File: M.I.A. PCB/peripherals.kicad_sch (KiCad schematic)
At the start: 69 parts, among them J10 Conn_01x03, J11 Conn_01x03, J12 MSD-4-A, J13 Conn_01x04_Socket, J14 Conn_01x03, J15 Conn_01x03, J16 Conn_01x03, J17 Conn_01x03, J18 Conn_01x04_Socket, J19 Conn_01x04_Socket, J20 Screw_Terminal_01x02, J21 Screw_Terminal_01x02, J22 Screw_Terminal_01x02, J23 Screw_Terminal_01x02, J24 Conn_01x04_Socket, J25 Conn_01x08_Socket, J26 Conn_01x04_Socket, J27 Conn_01x02_Socket, J28 Conn_01x04_Socket, J29 Conn_01x02_Socket, J30 Conn_01x02_Socket, J31 Conn_01x02_Socket, J32 Screw_Terminal_01x02, J33 Screw_Terminal_01x02, J6 Conn_01x04_Socket, J7 Conn_01x03, J8 Conn_01x03, J9 Conn_01x04_Socket, Q1 AO3400A, Q2 AO3400A, Q3 AO3400A, Q4 AO3400A, U15 74AHC541

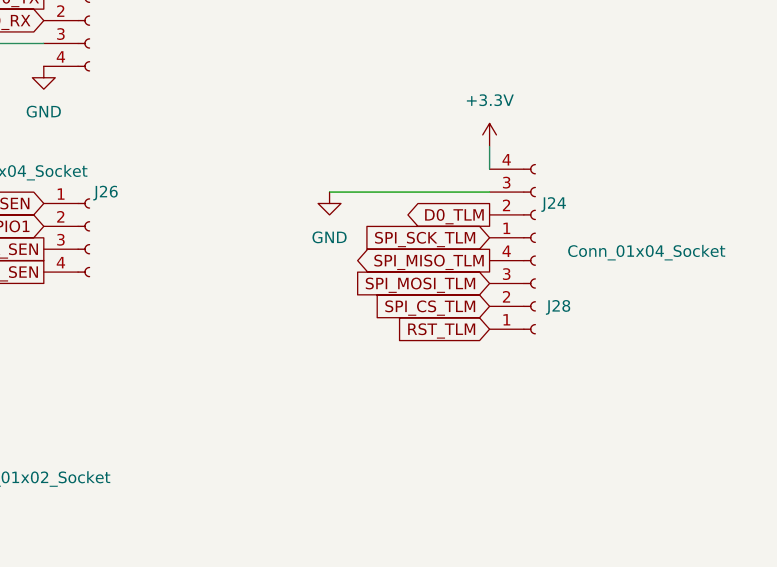
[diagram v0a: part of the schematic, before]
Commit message: Final Fixes, impedances, silkscreen etc
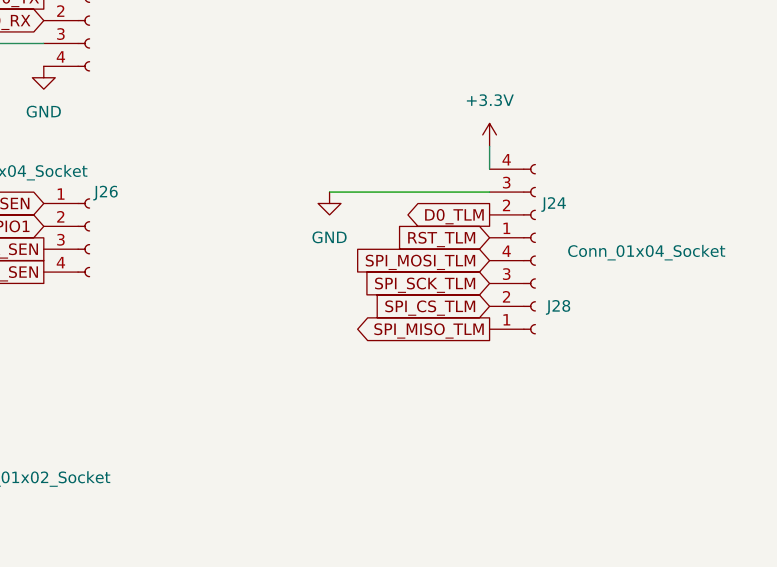
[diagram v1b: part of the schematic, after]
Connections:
- net RST_TLM: now also J24.1 (Pin_1); no longer J28.1 (Pin_1)
- net SPI_MISO_TLM: now also J28.1 (Pin_1); no longer J28.4 (Pin_4)
- net SPI_MOSI_TLM: now also J28.4 (Pin_4); no longer J28.3 (Pin_3)
- net SPI_SCK_TLM: now also J28.3 (Pin_3); no longer J24.1 (Pin_1)
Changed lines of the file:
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@@
 	(global_label "SPI_SCK_TLM"
 		(shape input)
-		(at 313.69 130.81 180)
-		(fields_autoplaced yes)
-		(effects
-			(font
-				(size 1.27 1.27)
-			)
-			(justify right)
-		)
-		(property "Intersheetrefs" "${INTERSHEET_REFS}"
-			(at 298.4887 130.81 0)
+		(at 313.69 135.89 180)
+		(fields_autoplaced yes)
+		(effects
+			(font
+				(size 1.27 1.27)
+			)
+			(justify right)
+		)
+		(property "Intersheetrefs" "${INTERSHEET_REFS}"
+			(at 299.7587 135.89 0)
 			(effects
 				(font
@@
 	(global_label "SPI_MISO_TLM"
 		(shape output)
-		(at 313.69 133.35 180)
-		(fields_autoplaced yes)
-		(effects
-			(font
-				(size 1.27 1.27)
-			)
-			(justify right)
-		)
-		(property "Intersheetrefs" "${INTERSHEET_REFS}"
-			(at 297.642 133.35 0)
+		(at 313.69 140.97 180)
+		(fields_autoplaced yes)
+		(effects
+			(font
+				(size 1.27 1.27)
+			)
+			(justify right)
+		)
+		(property "Intersheetrefs" "${INTERSHEET_REFS}"
+			(at 297.642 140.97 0)
 			(effects
 				(font
@@
 	(global_label "SPI_MOSI_TLM"
 		(shape input)
-		(at 313.69 135.89 180)
-		(fields_autoplaced yes)
-		(effects
-			(font
-				(size 1.27 1.27)
-			)
-			(justify right)
-		)
-		(property "Intersheetrefs" "${INTERSHEET_REFS}"
-			(at 297.642 135.89 0)
+		(at 313.69 133.35 180)
+		(fields_autoplaced yes)
+		(effects
+			(font
+				(size 1.27 1.27)
+			)
+			(justify right)
+		)
+		(property "Intersheetrefs" "${INTERSHEET_REFS}"
+			(at 302.843 133.35 0)
 			(effects
 				(font
@@
 	(global_label "RST_TLM"
 		(shape input)
-		(at 313.69 140.97 180)
-		(fields_autoplaced yes)
-		(effects
-			(font
-				(size 1.27 1.27)
-			)
-			(justify right)
-		)
-		(property "Intersheetrefs" "${INTERSHEET_REFS}"
-			(at 302.843 140.97 0)
+		(at 313.69 130.81 180)
+		(fields_autoplaced yes)
+		(effects
+			(font
+				(size 1.27 1.27)
+			)
+			(justify right)
+		)
+		(property "Intersheetrefs" "${INTERSHEET_REFS}"
+			(at 298.4887 130.81 0)
 			(effects
 				(font
@@
 		)
 		(property "Intersheetrefs" "${INTERSHEET_REFS}"
-			(at 299.7587 138.43 0)
-			(effects
-				(font
+			(at 297.642 138.43 0)
+			(effects
+				(font

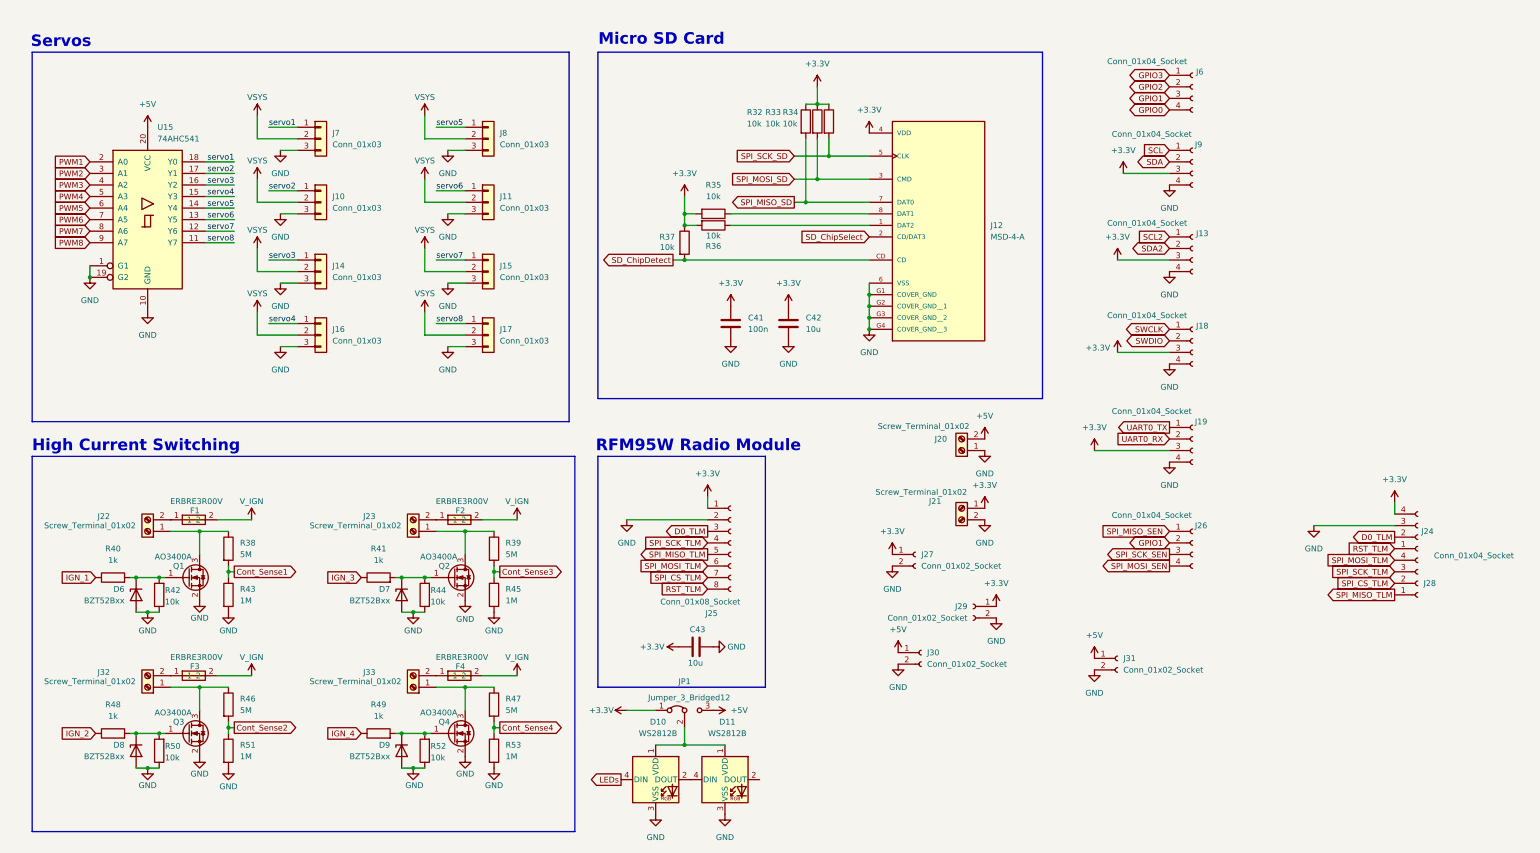
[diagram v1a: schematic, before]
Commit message: More Small Updates/Improvements
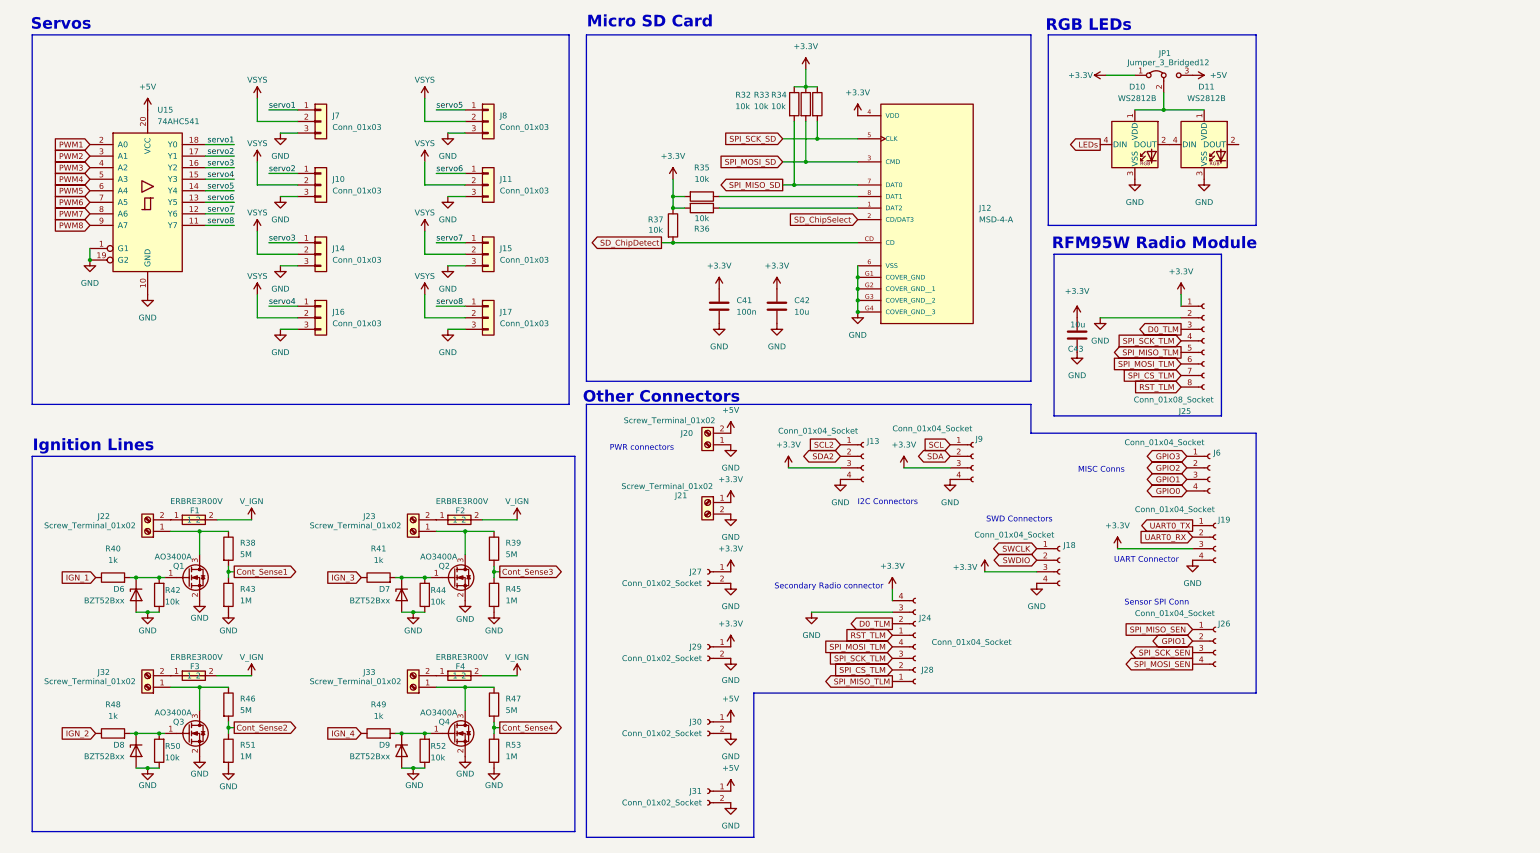
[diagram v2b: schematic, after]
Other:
- note added: "I2C Connectors"
- note added: "Ignition Lines"
- note added: "MISC Conns"
- note added: "Other Connectors"
- note added: "PWR connectors"
- note added: "RGB LEDs"
- note added: "SWD Connectors"
- note added: "Secondary Radio connector"
- note added: "Sensor SPI Conn"
- note added: "UART Connector"
- note removed: "High Current Switching"
- moved on the sheet: C41, C42, C43, D10, D11, J10, J11, J12, J13, J14, J15, J16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

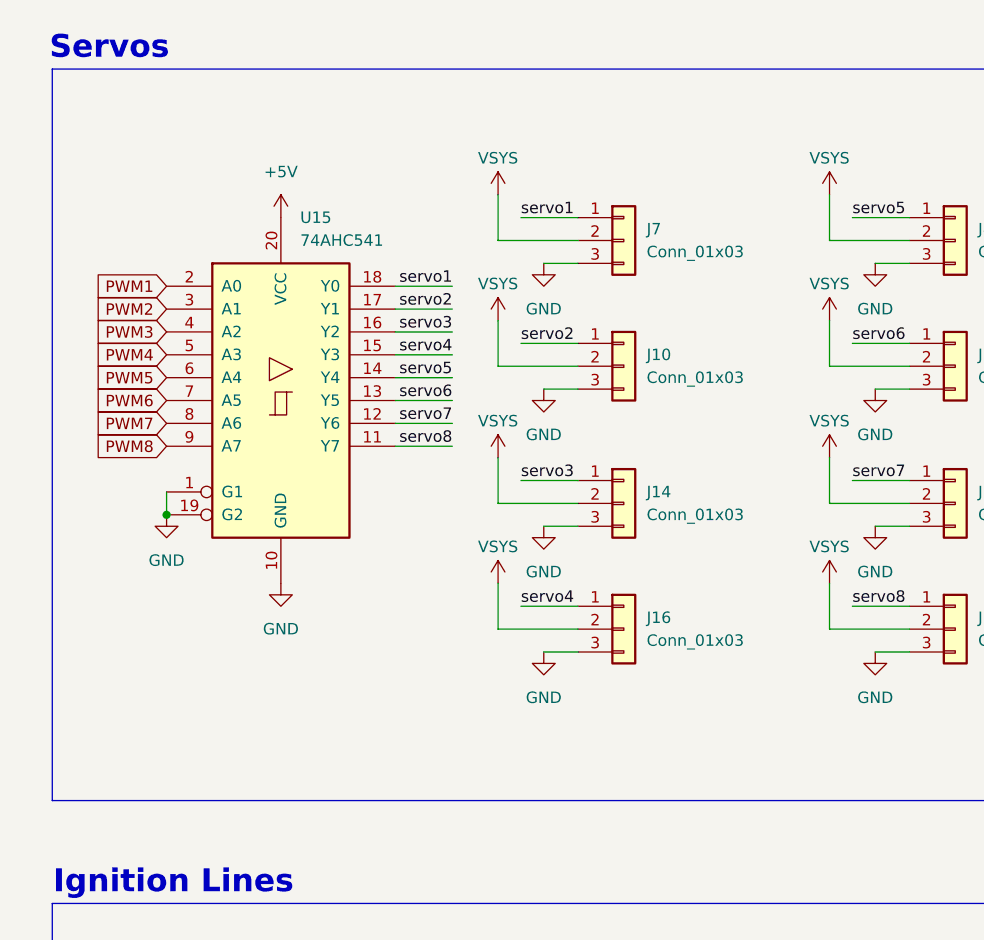
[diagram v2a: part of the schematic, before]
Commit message: Likely Final PCB
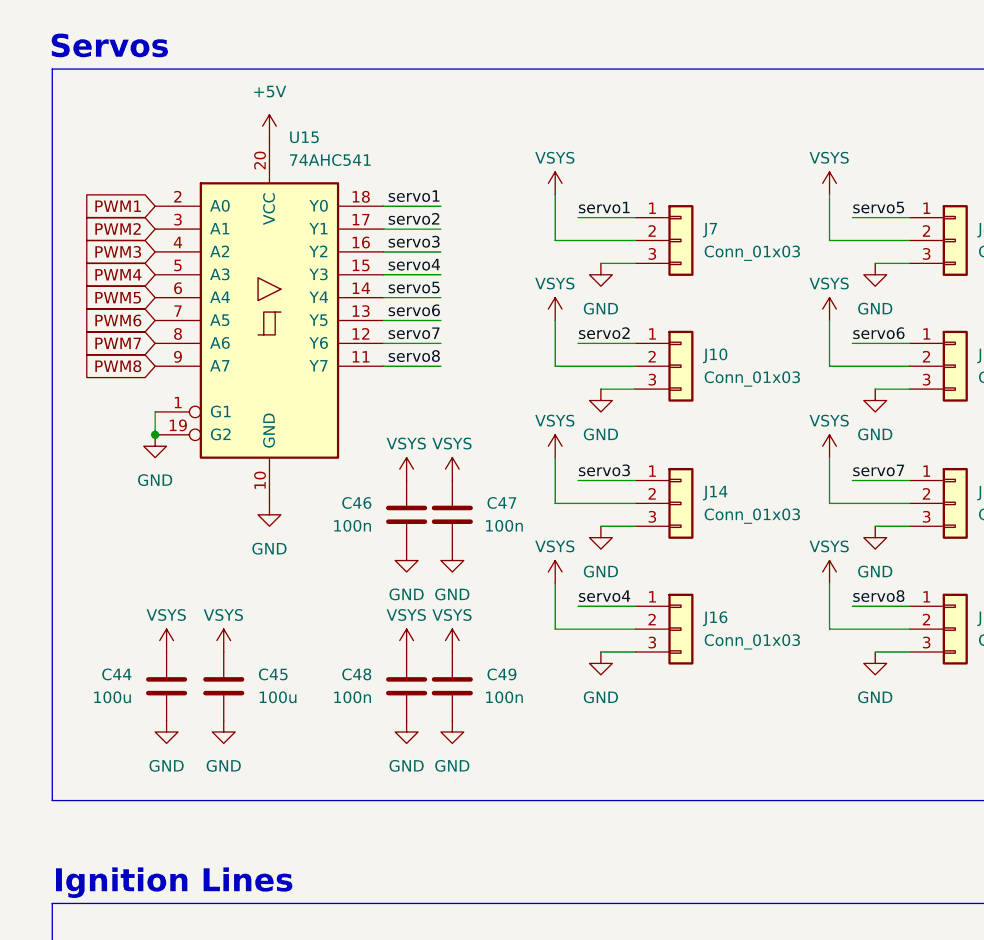
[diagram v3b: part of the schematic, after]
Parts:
- added C44, C45: 100u, Capacitor_THT:C_Radial_D5.0mm_H11.0mm_P2.00mm, symbol Device:C
- added C46, C47, C48, C49: 100n, Capacitor_SMD:C_0603_1608Metric, symbol Device:C
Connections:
- net GND: now also C44.2, C45.2, C46.2, C47.2, C48.2, C49.2
- net VSYS: now also C44.1, C45.1, C46.1, C47.1, C48.1, C49.1
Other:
- moved on the sheet: J10, J14, J16, J7, U15
